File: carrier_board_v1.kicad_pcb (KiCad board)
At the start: 2 copper layers, 40.1 x 55.1 mm, 31 parts, among them J1 B2B-PH-SM4-TB_LF__SN_, J3 54548-2271, J4 USB4105-GF-A, J6 USB4105-GF-A, J7 Conn_01x12_Pin, Q1 DMP3013SFV, U1 BQ25302RTER, U3 TPD2EUSB30, U5 TPS613222ADBZ

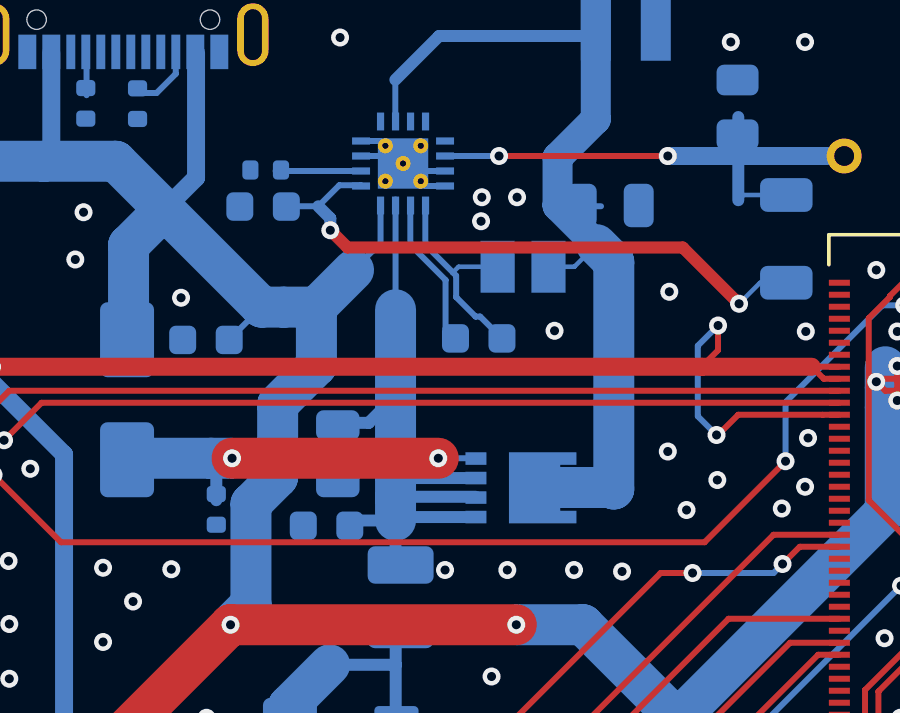
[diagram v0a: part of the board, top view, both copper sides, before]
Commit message: -
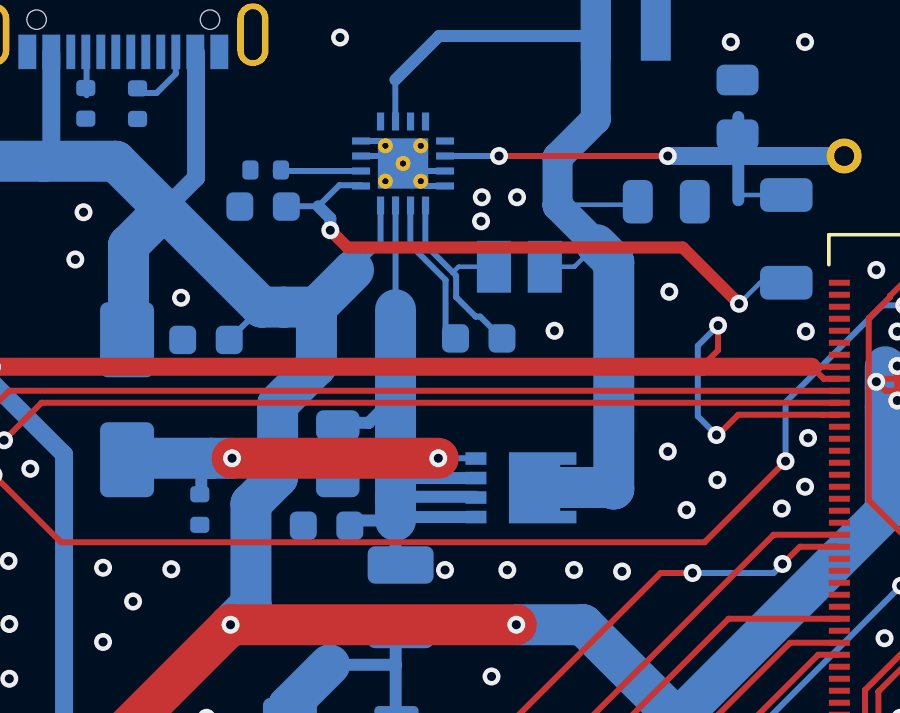
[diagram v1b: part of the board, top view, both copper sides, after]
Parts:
- moved C6 1.87 mm to (156.2, 91.0)
- moved R5 0.55 mm to (140.6, 101.3)
- moved L2 0.12 mm to (151.3, 93.2)
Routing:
- net Net-(Q1-D): track 33.4 -> 34.7 mm
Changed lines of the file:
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@@
   )
   (footprint "Resistor_SMD:R_0402_1005Metric" (layer "B.Cu")
-    (at 141.15 101.255 90)
+    (at 140.6 101.26 90)
     (descr "Resistor SMD 0402 (1005 Metric), square (rectangular) end terminal, IPC_7351 nominal, (Body size source: IPC-SM-782 page 72, https://www.pcb-3d.com/wordpress/wp-content/uploads/ipc-sm-782a_amendment_1_and_2.pdf), generated with kicad-footprint-generator")
     (tags "resistor")
@@
     (property "ki_keywords" "R res resistor")
     (attr smd)
-    (fp_text reference "R5" (at -0.7768 -1.3484) (layer "B.SilkS")
+    (fp_text reference "R5" (at -0.59 -1.5) (layer "B.SilkS")
         (effects (font (size 1 1) (thickness 0.15)) (justify mirror))
     )
@@
   )
   (footprint "Capacitor_SMD:C_0805_2012Metric" (layer "B.Cu")
-    (at 154.28 91.125)
+    (at 156.15 91)
     (descr "Capacitor SMD 0805 (2012 Metric), square (rectangular) end terminal, IPC_7351 nominal, (Body size source: IPC-SM-782 page 76, https://www.pcb-3d.com/wordpress/wp-content/uploads/ipc-sm-782a_amendment_1_and_2.pdf, https://docs.google.com/spreadsheets/d/1BsfQQcO9C6DZCsRaXUlFlo91Tg2WpOkGARC1WS5S8t0/edit?usp=sharing), generated with kicad-footprint-generator")
     (tags "capacitor")
@@
   )
   (footprint "MAKK2016T1R0M:INDC2016X100N" (layer "B.Cu")
-    (at 151.3752 93.1672)
+    (at 151.253 93.1672)
     (property "Sheetfile" "cm4-gpio.kicad_sch")
     (property "Sheetname" "CM4 GPIO and power pins")
@@
   (segment (start 160.15 93.7) (end 159.275 93.7) (width 0.1524) (layer "B.Cu") (net 6))
   (segment (start 152.575 91.15) (end 152.525 91.1) (width 0.2) (layer "B.Cu") (net 7))
+  (segment (start 155.2 91) (end 155.1 91.1) (width 0.1524) (layer "B.Cu") (net 7))
   (segment (start 152.525 91.1332) (end 152.525 91.1) (width 1) (layer "B.Cu") (net 7))
   (segment (start 147.1175 88.31) (end 147.1175 86.935) (width 0.2) (layer "B.Cu") (net 7))
@@
   (segment (start 153.0858 93.1672) (end 153.8224 92.4306) (width 0.1524) (layer "B.Cu") (net 7))
   (segment (start 152.2222 93.1672) (end 153.0858 93.1672) (width 0.1524) (layer "B.Cu") (net 7))
-  (segment (start 153.975 91.15) (end 152.575 91.15) (width 0.2) (layer "B.Cu") (net 7))
+  (segment (start 155.1 91.1) (end 152.525 91.1) (width 0.1524) (layer "B.Cu") (net 7))
   (segment (start 154.4 100.575) (end 154.35 100.525) (width 1.36703) (layer "B.Cu") (net 7))
   (segment (start 154.4 93.0082) (end 154.4 100.575) (width 1.36703) (layer "B.Cu") (net 7))
@@
   (via (at 141.675 99.55) (size 0.6) (drill 0.3) (layers "F.Cu" "B.Cu") (net 9))
   (via (at 148.55 99.55) (size 0.6) (drill 0.3) (layers "F.Cu" "B.Cu") (net 9))
-  (segment (start 141.15 99.725) (end 140.975 99.55) (width 0.4) (layer "B.Cu") (net 9))
+  (segment (start 140.65 99.875) (end 140.975 99.55) (width 0.4) (layer "B.Cu") (net 9))
   (segment (start 140.975 99.55) (end 138.25 99.55) (width 1.36703) (layer "B.Cu") (net 9))
   (segment (start 149.85 99.55) (end 148.55 99.55) (width 0.2) (layer "B.Cu") (net 9))
   (segment (start 138.25 99.55) (end 138.225 99.525) (width 1.36703) (layer "B.Cu") (net 9))
   (segment (start 141.675 99.55) (end 140.975 99.55) (width 1.36703) (layer "B.Cu") (net 9))
-  (segment (start 141.15 100.95) (end 141.15 99.725) (width 0.4) (layer "B.Cu") (net 9))
+  (segment (start 140.65 100.745) (end 140.65 99.875) (width 0.4) (layer "B.Cu") (net 9))
   (segment (start 147.13 105.4222) (end 147.2946 105.2576) (width 0.4) (layer "B.Cu") (net 10))
   (segment (start 147.13 106.435) (end 144.93 106.435) (width 0.4) (layer "B.Cu") (net 10))

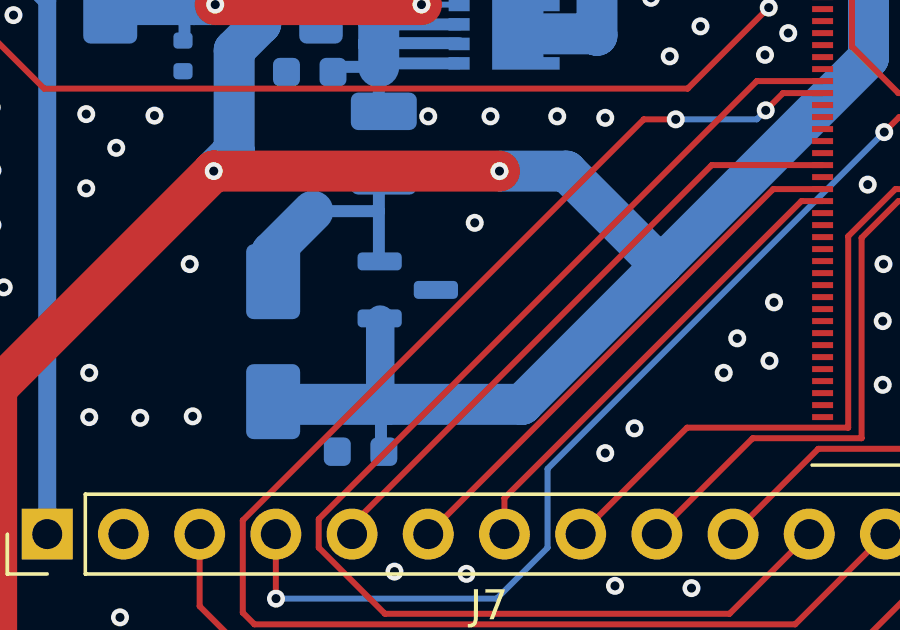
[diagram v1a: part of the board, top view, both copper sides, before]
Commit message: -
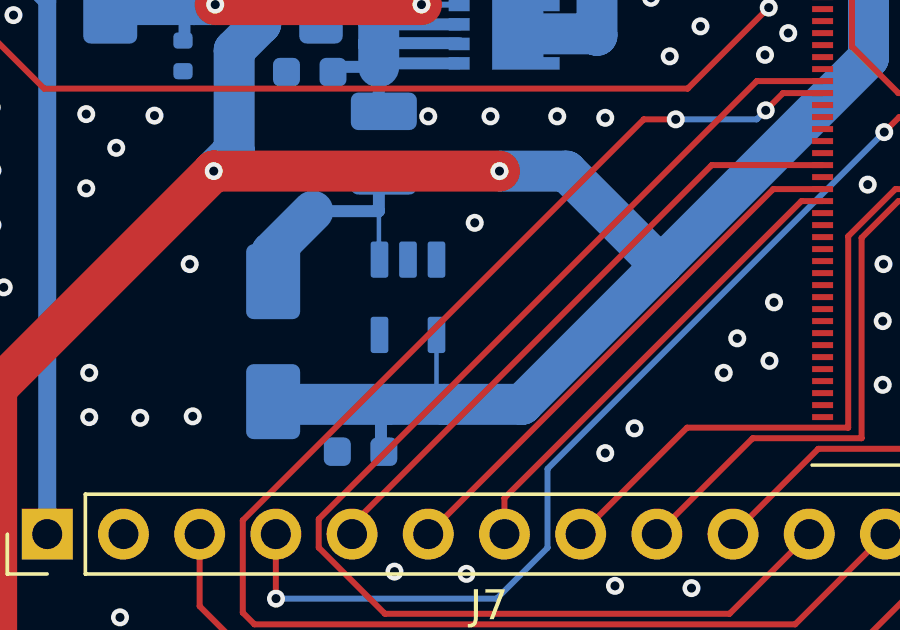
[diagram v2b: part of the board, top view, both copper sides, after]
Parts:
- removed U5: TPS613222ADBZ, Package_TO_SOT_SMD:SOT-23
- added U2: TPS613222ADBVT, TPS613222ADBVT:SOT95P280X145-5N, B.Cu at (148.1, 109.3)
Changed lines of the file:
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@@
-    )
-  )
-  (footprint "Package_TO_SOT_SMD:SOT-23" (layer "B.Cu")
-    (at 148.0925 109.06)
-    (descr "SOT, 3 Pin (https://www.jedec.org/system/files/docs/to-236h.pdf variant AB), generated with kicad-footprint-generator ipc_gullwing_generator.py")
-    (tags "SOT TO_SOT_SMD")
-    (property "Sheetfile" "cm4-gpio.kicad_sch")
-    (property "Sheetname" "CM4 GPIO and power pins")
-    (property "ki_description" "1.8A Step-Up Converter, 5V Output Voltage, 0.9-5.5V Input Voltage, SOT-23")
-    (property "ki_keywords" "Boost converter")
-    (attr smd)
-    (fp_text reference "U5" (at 2.8075 -0.01) (layer "B.SilkS")
-        (effects (font (size 1 1) (thickness 0.15)) (justify mirror))
-    )
-    (fp_text value "TPS613222ADBZ" (at 0 -2.4) (layer "B.Fab")
-        (effects (font (size 1 1) (thickness 0.15)) (justify mirror))
-    )
-    (fp_text user "${REFERENCE}" (at 0 0) (layer "B.Fab")
-        (effects (font (size 0.32 0.32) (thickness 0.05)) (justify mirror))
-    )
-    (fp_line (start 0 -1.56) (end -0.65 -1.56)
-      (stroke (width 0.12) (type solid)) (layer "B.SilkS"))
-    (fp_line (start 0 -1.56) (end 0.65 -1.56)
-      (stroke (width 0.12) (type solid)) (layer "B.SilkS"))
-    (fp_line (start 0 1.56) (end -1.675 1.56)
-      (stroke (width 0.12) (type solid)) (layer "B.SilkS"))
-    (fp_line (start 0 1.56) (end 0.65 1.56)
-      (stroke (width 0.12) (type solid)) (layer "B.SilkS"))
-    (fp_line (start -1.92 -1.7) (end 1.92 -1.7)
-      (stroke (width 0.05) (type solid)) (layer "B.CrtYd"))
-    (fp_line (start -1.92 1.7) (end -1.92 -1.7)
-      (stroke (width 0.05) (type solid)) (layer "B.CrtYd"))
-    (fp_line (start 1.92 -1.7) (end 1.92 1.7)
-      (stroke (width 0.05) (type solid)) (layer "B.CrtYd"))
-    (fp_line (start 1.92 1.7) (end -1.92 1.7)
-      (stroke (width 0.05) (type solid)) (layer "B.CrtYd"))
-    (fp_line (start -0.65 -1.45) (end -0.65 1.125)
-      (stroke (width 0.1) (type solid)) (layer "B.Fab"))
-    (fp_line (start -0.65 1.125) (end -0.325 1.45)
-      (stroke (width 0.1) (type solid)) (layer "B.Fab"))
-    (fp_line (start -0.325 1.45) (end 0.65 1.45)
-      (stroke (width 0.1) (type solid)) (layer "B.Fab"))
-    (fp_line (start 0.65 -1.45) (end -0.65 -1.45)
-      (stroke (width 0.1) (type solid)) (layer "B.Fab"))
-    (fp_line (start 0.65 1.45) (end 0.65 -1.45)
-      (stroke (width 0.1) (type solid)) (layer "B.Fab"))
-    (pad "1" smd roundrect (at -0.9375 0.95) (size 1.475 0.6) (layers "B.Cu" "B.Paste" "B.Mask") (roundrect_rratio 0.25)
-      (net 1 "+5V") (pinfunction "VOUT") (pintype "power_out"))
-    (pad "2" smd roundrect (at -0.9375 -0.95) (size 1.475 0.6) (layers "B.Cu" "B.Paste" "B.Mask") (roundrect_rratio 0.25)
-      (net 10 "Net-(D2-A)") (pinfunction "SW") (pintype "power_in"))
-    (pad "3" smd roundrect (at 0.9375 0) (size 1.475 0.6) (layers "B.Cu" "B.Paste" "B.Mask") (roundrect_rratio 0.25)
-      (net 2 "GND") (pinfunction "GND") (pintype "power_in"))
-    (model "${KICAD6_3DMODEL_DIR}/Package_TO_SOT_SMD.3dshapes/SOT-23.wrl"
-      (offset (xyz 0 0 0))
-      (scale (xyz 1 1 1))
-      (rotate (xyz 0 0 0))
     )
   )
@@
     )
   )
+  (footprint "TPS613222ADBVT:SOT95P280X145-5N" (layer "B.Cu")
+    (at 148.1 109.305 -90)
+    (property "Sheetfile" "cm4-gpio.kicad_sch")
+    (property "Sheetname" "CM4 GPIO and power pins")
+    (attr smd)
+    (fp_text reference "U2" (at -0.06 2.508 90) (layer "B.SilkS")
+        (effects (font (size 0.8 0.8) (thickness 0.15)) (justify mirror))
+    )
+    (fp_text value "TPS613222ADBVT" (at 5.528 -2.508 90) (layer "B.Fab")
+        (effects (font (size 0.8 0.8) (thickness 0.15)) (justify mirror))
+    )
+    (fp_line (start -0.33 1.45) (end 0.33 1.45)
+      (stroke (width 0.127) (type solid)) (layer "B.SilkS"))
+    (fp_line (start 0.33 -1.45) (end -0.33 -1.45)
+      (stroke (width 0.127) (type solid)) (layer "B.SilkS"))
+    (fp_line (start 0.8 0.335) (end 0.8 -0.335)
+      (stroke (width 0.127) (type solid)) (layer "B.SilkS"))
+    (fp_circle (center -2.41 1.05) (end -2.31 1.05)
+      (stroke (width 0.2) (type solid)) (fill none) (layer "B.SilkS"))
+    (fp_line (start -2.11 -1.7) (end -2.11 1.7)
+      (stroke (width 0.05) (type solid)) (layer "B.CrtYd"))
+    (fp_line (start -2.11 1.7) (end 2.11 1.7)
+      (stroke (width 0.05) (type solid)) (layer "B.CrtYd"))
+    (fp_line (start 2.11 -1.7) (end -2.11 -1.7)
+      (stroke (width 0.05) (type solid)) (layer "B.CrtYd"))
+    (fp_line (start 2.11 1.7) (end 2.11 -1.7)
+      (stroke (width 0.05) (type solid)) (layer "B.CrtYd"))
+    (fp_line (start -0.8 -1.45) (end -0.8 1.45)
+      (stroke (width 0.127) (type solid)) (layer "B.Fab"))
+    (fp_line (start -0.8 1.45) (end 0.8 1.45)
+      (stroke (width 0.127) (type solid)) (layer "B.Fab"))
+    (fp_line (start 0.8 -1.45) (end -0.8 -1.45)
+      (stroke (width 0.127) (type solid)) (layer "B.Fab"))
+    (fp_line (start 0.8 1.45) (end 0.8 -1.45)
+      (stroke (width 0.127) (type solid)) (layer "B.Fab"))
+    (fp_circle (center -2.41 1.05) (end -2.31 1.05)
+      (stroke (width 0.2) (type solid)) (fill none) (layer "B.Fab"))
+    (pad "1" smd roundrect (at -1.255 0.95 270) (size 1.21 0.59) (layers "B.Cu" "B.Paste" "B.Mask") (roundrect_rratio 0.15)
+      (net 10 "Net-(D2-A)") (pinfunction "SW") (pintype "bidirectional"))
+    (pad "2" smd roundrect (at -1.255 0 270) (size 1.21 0.59) (layers "B.Cu" "B.Paste" "B.Mask") (roundrect_rratio 0.15)
+      (net 2 "GND") (pinfunction "GND") (pintype "power_in"))
+    (pad "3" smd roundrect (at -1.255 -0.95 270) (size 1.21 0.59) (layers "B.Cu" "B.Paste" "B.Mask") (roundrect_rratio 0.15))
+    (pad "4" smd roundrect (at 1.255 -0.95 270) (size 1.21 0.59) (layers "B.Cu" "B.Paste" "B.Mask") (roundrect_rratio 0.15)
+      (net 1 "+5V") (pinfunction "VOUT") (pintype "output"))
+    (pad "5" smd roundrect (at 1.255 0.95 270) (size 1.21 0.59) (layers "B.Cu" "B.Paste" "B.Mask") (roundrect_rratio 0.15))
+  )
   (footprint "Package_SON:Diodes_PowerDI3333-8" (layer "B.Cu")
     (at 151.305 100.535)
@@
   (segment (start 142.6625 94.5125) (end 143.4 94.5125) (width 1.36703) (layer "B.Cu") (net 1))
   (segment (start 141.2649 124.2149) (end 140.71025 123.66025) (width 0.6) (layer "B.Cu") (net 1))
-  (segment (start 147.4 112.875) (end 151.9 112.875) (width 1.36703) (layer "B.Cu") (net 1))
   (segment (start 147.2 114.525) (end 147.2 113.075) (width 0.4) (layer "B.Cu") (net 1))
   (segment (start 143.5 94.6125) (end 143.4 94.5125) (width 0.2) (layer "B.Cu") (net 1))
@@
   (segment (start 140.475 90.2) (end 139.4125 91.2625) (width 0.6) (layer "B.Cu") (net 1))
   (segment (start 140.8948 126.044439) (end 141.2649 125.674339) (width 0.6) (layer "B.Cu") (net 1))
+  (segment (start 149.05 112.625) (end 149.3 112.875) (width 0.1524) (layer "B.Cu") (net 1))
   (segment (start 140.475 86.025) (end 140.475 90.2) (width 0.6) (layer "B.Cu") (net 1))
   (segment (start 151.9 112.875) (end 156.525 108.25) (width 1.36703) (layer "B.Cu") (net 1))
@@
   (segment (start 163.45 101.325) (end 163.45 97.85) (width 1.36703) (layer "B.Cu") (net 1))
   (segment (start 138.225 92.45) (end 139.4125 91.2625) (width 1.36703) (layer "B.Cu") (net 1))
-  (segment (start 147.175 110.05) (end 147.175 112.65) (width 0.95) (layer "B.Cu") (net 1))
+  (segment (start 147.4 112.875) (end 149.3 112.875) (width 1.36703) (layer "B.Cu") (net 1))
   (segment (start 145.725 93.275) (end 144.4875 94.5125) (width 1.36703) (layer "B.Cu") (net 1))
   (segment (start 140.71025 123.66025) (end 140.28975 123.66025) (width 0.6) (layer "B.Cu") (net 1))
@@
   (segment (start 143.19443 97.75557) (end 143.19443 100.179369) (width 1.36703) (layer "B.Cu") (net 1))
   (segment (start 153.375 105.1) (end 151.15 105.1) (width 1.36703) (layer "B.Cu") (net 1))
+  (segment (start 149.3 112.875) (end 151.9 112.875) (width 1.36703) (layer "B.Cu") (net 1))
   (segment (start 137.8 89.65) (end 139.4125 91.2625) (width 1.36703) (layer "B.Cu") (net 1))
+  (segment (start 149.05 110.56) (end 149.05 112.625) (width 0.1524) (layer "B.Cu") (net 1))
   (segment (start 138.225 95.65) (end 138.225 92.45) (width 1.36703) (layer "B.Cu") (net 1))
   (segment (start 141.2649 125.674339) (end 141.2649 124.2149) (width 0.6) (layer "B.Cu") (net 1))
@@
   (segment (start 147.13 105.4222) (end 147.2946 105.2576) (width 0.4) (layer "B.Cu") (net 10))
   (segment (start 147.13 106.435) (end 144.93 106.435) (width 0.4) (layer "B.Cu") (net 10))
-  (segment (start 147.13 106.435) (end 147.13 108.01) (width 0.4) (layer "B.Cu") (net 10))
+  (segment (start 147.15 108.05) (end 147.13 108.03) (width 0.1524) (layer "B.Cu") (net 10))
+  (segment (start 147.13 108.03) (end 147.13 106.435) (width 0.1524) (layer "B.Cu") (net 10))
   (segment (start 147.13 106.435) (end 147.13 105.4222) (width 0.4) (layer "B.Cu") (net 10))
   (segment (start 144.93 106.435) (end 143.555 107.81) (width 1.36703) (layer "B.Cu") (net 10))
